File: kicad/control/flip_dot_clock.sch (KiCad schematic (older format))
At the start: 12 parts, among them U1 NUCLEO-F303K8-HEADER, U10 Small_7_Seg_FlipDot_Module, U2 SLC03B-05, U3 NCV7719, U4 Small_7_Seg_FlipDot_Module, U5 NCV7719, U6 Small_7_Seg_FlipDot_Module, U7 NCV7719, U8 Small_7_Seg_FlipDot_Module, U9 NCV7719

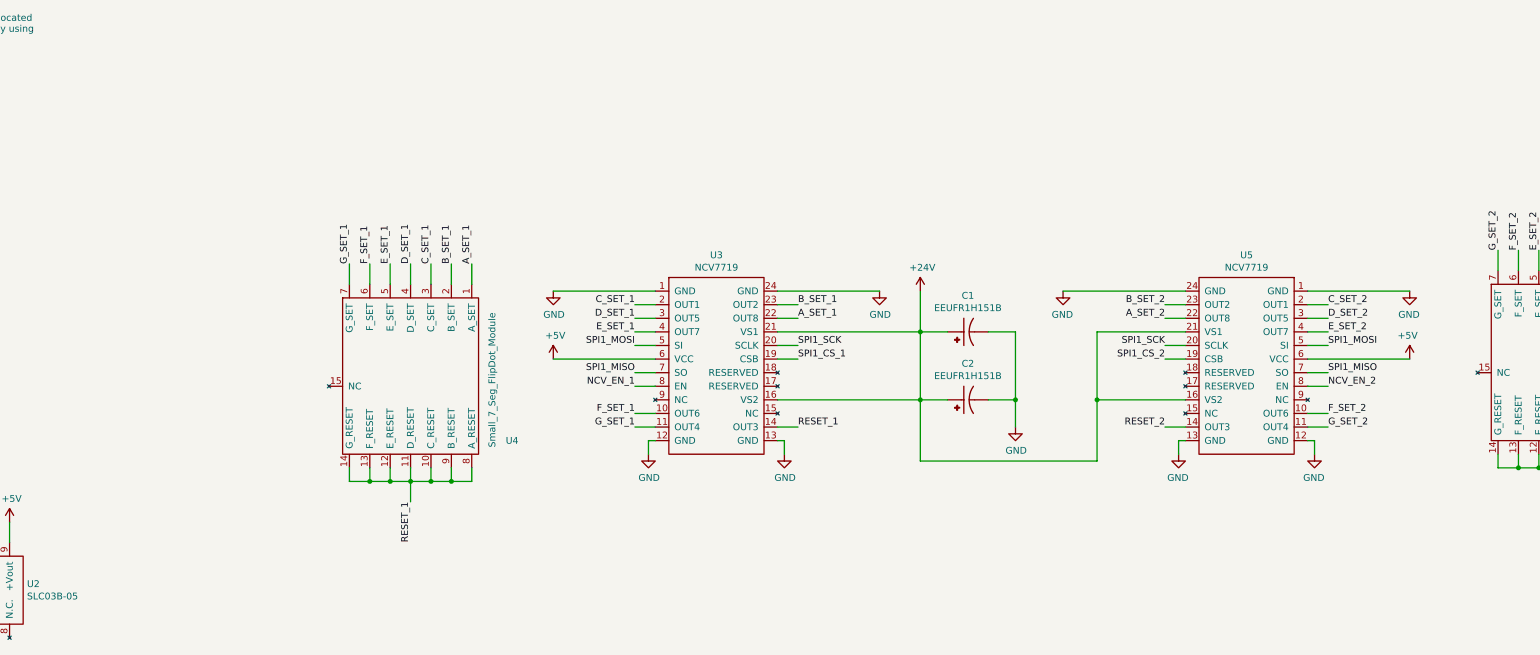
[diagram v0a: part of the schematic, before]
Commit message: update parts
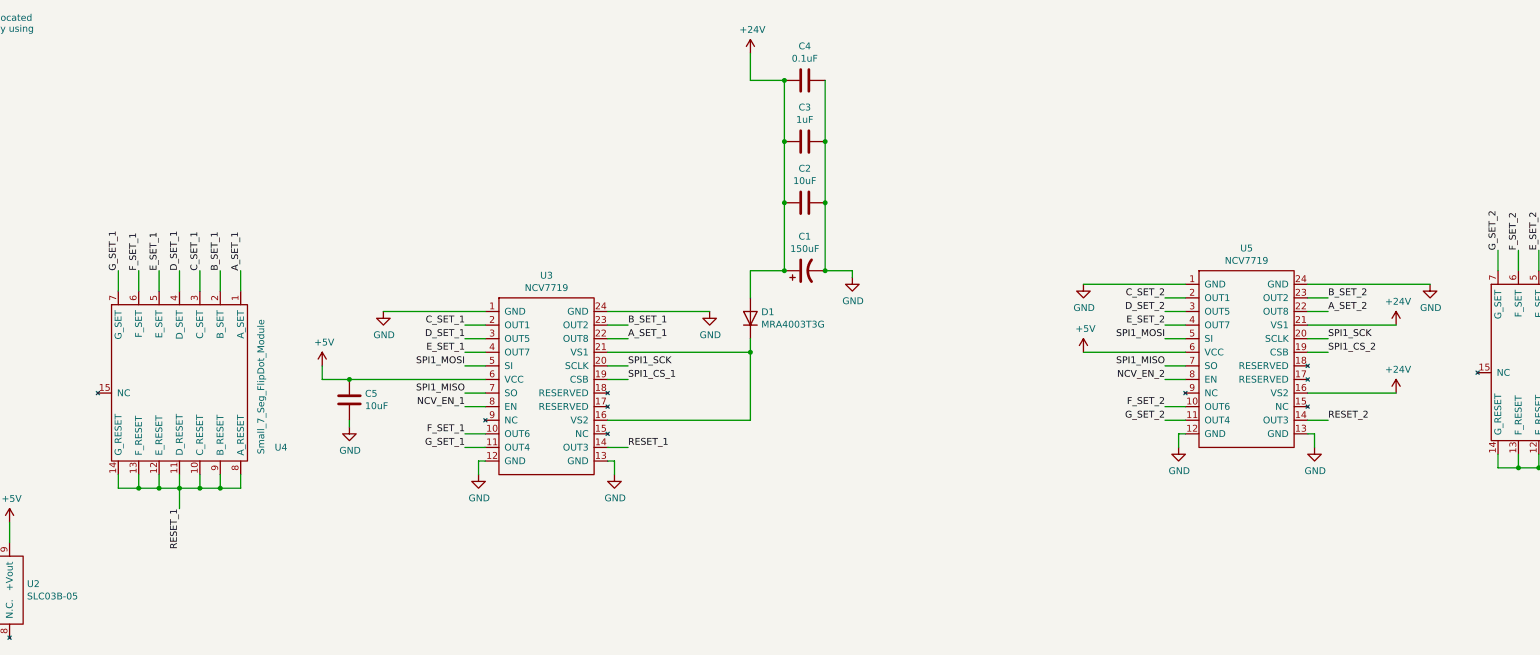
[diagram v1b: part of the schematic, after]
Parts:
- removed C1, C2: EEUFR1H151B, CAPPRD500W60D1000H1250, symbol EEUFR1H151B:EEUFR1H151B
- added C1: 150uF, Capacitor_THT:CP_Radial_D10.0mm_P5.00mm, symbol Device:CP1
- added C2: 10uF, Capacitor_SMD:C_1206_3216Metric, symbol Device:C
- added C3: 1uF, Capacitor_SMD:C_1206_3216Metric, symbol Device:C
- added C4: 0.1uF, Capacitor_SMD:C_1206_3216Metric, symbol Device:C
- added C5: 10uF, symbol Device:C
- added D1: MRA4003T3G, Diode_SMD:D_SMA, symbol Diode:MRA4003T3G
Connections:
- net +24V: now also C1.1, C2.2, C3.2, C4.2, D1.2 (A); no longer U3.16 (VS2), U3.21 (VS1)
- net +5V: now also C5.1
- net GND: now also C1.2, C2.1, C3.1, C4.1, C5.2
- new net: D1.1 (K), U3.16 (VS2), U3.21 (VS1)
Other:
- moved on the sheet: U3, U4, U5
